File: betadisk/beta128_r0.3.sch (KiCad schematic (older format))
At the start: 85 parts, among them J1 ZX_Spectrum_Connector_GENERIC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, J2 Conn_02x17_Odd_Even, Q1 BC639, SW1 SW_DIP_x02, U10 74LS174, U11 74LS367, U12 FDC_MB8877, U13 74LS14, U14 74LS139, U15 74LS06, U16 74LS74, U17 74LS161, U18 74LS161, U19 74LS00, U21 L7805, U22 GAL22V10, U3 W27C512, U4 74LS32, U6 74LS30, U7 74LS123, U8 74LS74, U9 74LS07, U99 74LS245, Y1 8.000Mhz

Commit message: schematic in pdf
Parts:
- removed C1, C103, C104, C106, C107, C108, C109, C110, C111, C112, C113, C114, C115, C116, C117, C118, C119, C122, C199, C4, C5: 100n, Capacitor_THT:C_Disc_D5.0mm_W2.5mm_P5.00mm, symbol Device:C
- removed C2, C3: 220u/16 V, Capacitor_THT:CP_Radial_D7.5mm_P2.50mm, symbol Device:CP
- removed C6: 10u/16 V, Capacitor_THT:CP_Radial_D7.5mm_P2.50mm, symbol Device:CP
- removed C7: 33p, Capacitor_THT:C_Disc_D5.0mm_W2.5mm_P5.00mm, symbol Device:C
- removed C8: 100u/16 V, Capacitor_THT:CP_Radial_D7.5mm_P2.50mm, symbol Device:CP
- removed D1, D5: LED, LED_THT:LED_D5.0mm, symbol Device:LED
- removed D15: BAT42, Diode_THT:D_DO-35_SOD27_P7.62mm_Horizontal, symbol Diode:BAT42
- removed D7, D8, D9: 1N4148, Diode_THT:D_DO-35_SOD27_P7.62mm_Horizontal, symbol Diode:1N4148
- removed H1, H2, H3, H4: MountingHole, MountingHole:MountingHole_3mm, symbol Mechanical:MountingHole
- removed J1: ZX_Spectrum_Connector_GENERIC_SORTED, SINCLAIR:ZX_EDGE_90extend, symbol 8bits:ZX_Spectrum_Connector_GENERIC_SORTED
- removed J2: Conn_02x17_Odd_Even, Connector_PinHeader_2.54mm:PinHeader_2x17_P2.54mm_Vertical, symbol Connector_Generic:Conn_02x17_Odd_Even
- removed JP2: Conn_01x03, Connector_PinHeader_2.54mm:PinHeader_1x03_P2.54mm_Vertical, symbol Connector_Generic:Conn_01x03
- removed JP3: a, Connector_PinHeader_2.54mm:PinHeader_2x02_P2.54mm_Vertical, symbol Connector_Generic:Conn_02x02_Odd_Even
- removed JP4: Conn_02x02_Odd_Even, Connector_PinHeader_2.54mm:PinHeader_2x02_P2.54mm_Vertical, symbol Connector_Generic:Conn_02x02_Odd_Even
- removed JP5: Conn_01x04_Male, Connector_PinHeader_2.54mm:PinHeader_1x05_P2.54mm_Vertical, symbol Connector:Conn_01x05_Male
- removed Q1: BC639, symbol Device:Q_NPN_ECB
- removed R1: 1k, Resistor_THT:R_Axial_DIN0207_L6.3mm_D2.5mm_P7.62mm_Horizontal, symbol Device:R
- removed R11, R12: 10K, Resistor_THT:R_Axial_DIN0207_L6.3mm_D2.5mm_P7.62mm_Horizontal, symbol Device:R
- removed R13, R14, R15, R16, R17, R3: 470, Resistor_THT:R_Axial_DIN0207_L6.3mm_D2.5mm_P7.62mm_Horizontal, symbol Device:R
- removed R18, R21, R22: 6k8, Resistor_THT:R_Axial_DIN0207_L6.3mm_D2.5mm_P7.62mm_Horizontal, symbol Device:R
- removed R19, R20: 2K2, Resistor_THT:R_Axial_DIN0207_L6.3mm_D2.5mm_P7.62mm_Horizontal, symbol Device:R
- removed R2, R5: 5k6, Resistor_THT:R_Axial_DIN0207_L6.3mm_D2.5mm_P7.62mm_Horizontal, symbol Device:R
- removed R6: 120k, Resistor_THT:R_Axial_DIN0207_L6.3mm_D2.5mm_P7.62mm_Horizontal, symbol Device:R
- removed R8, R9: 680, Resistor_THT:R_Axial_DIN0207_L6.3mm_D2.5mm_P7.62mm_Horizontal, symbol Device:R
- removed S1: 255SB, SINCLAIR:SW_C&K_710x-xx-xx-Z-_SPDT, symbol beta128_r0.3-rescue:255SB-dos_5-0x-eagle-import
- removed S2: 10-XX, Button_Switch_THT:SW_TH_Tactile_Omron_B3F-10xx, symbol beta128_r0.3-rescue:10-XX-dos_5-0x-eagle-import
- removed SW1: SW_DIP_x02, Button_Switch_THT:SW_DIP_SPSTx02_Slide_9.78x7.26mm_W7.62mm_P2.54mm, symbol Switch:SW_DIP_x02
- removed U10: 74LS174, Package_DIP:DIP-16_W7.62mm_LongPads, symbol 74xx:74LS174
- removed U11: 74LS367, Package_DIP:DIP-16_W7.62mm_LongPads, symbol 74xx:74LS367
- removed U12: FDC_MB8877, Package_DIP:DIP-40_W15.24mm_LongPads, symbol 8bits:FDC_MB8877
- removed U13: 74LS14, Package_DIP:DIP-14_W7.62mm_LongPads, symbol 74xx:74LS14
- removed U14: 74LS139, Package_DIP:DIP-16_W7.62mm_LongPads, symbol 74xx:74LS139
- removed U15: 74LS06, Package_DIP:DIP-14_W7.62mm_LongPads, symbol 74xx:74LS06
- removed U16, U8: 74LS74, Package_DIP:DIP-14_W7.62mm_LongPads, symbol 74xx:74LS74
- removed U17, U18: 74LS161, Package_DIP:DIP-16_W7.62mm_LongPads, symbol 74xx:74LS161
- removed U19: 74LS00, Package_DIP:DIP-14_W7.62mm_LongPads, symbol 74xx:74LS00
- removed U21: L7805, Package_TO_SOT_THT:TO-220-3_Vertical, symbol Regulator_Linear:L7805
- removed U22: GAL22V10, Package_DIP:DIP-24_W7.62mm_LongPads, symbol 8bits:GAL22V10
- removed U3: W27C512, Package_DIP:DIP-28_W15.24mm_LongPads, symbol 8bits:W27C512
- removed U4: 74LS32, Package_DIP:DIP-14_W7.62mm_LongPads, symbol 74xx:74LS32
- removed U6: 74LS30, Package_DIP:DIP-14_W7.62mm_LongPads, symbol 74xx:74LS30
- removed U7: 74LS123, Package_DIP:DIP-16_W7.62mm_LongPads, symbol 74xx:74LS123
- removed U9: 74LS07, Package_DIP:DIP-14_W7.62mm_LongPads, symbol 74xx:74LS07
- removed U99: 74LS245, Package_DIP:DIP-20_W7.62mm_LongPads, symbol 74xx:74LS245
- removed Y1: 8.000Mhz, Crystal:Crystal_HC18-U_Vertical, symbol Device:Crystal
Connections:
- net labels removed: +5V, +9V, 4Mhz, A0, A1, A10, A11, A12, A13, A14, A14+A15, A15, A2, A3, A4, A5, A6, A7, A8, A9, A[0...15], D'0, D'1, D'2, D'3, D'4, D'5, D'6, D'7, D'[0...7], D0, D1, D2, D3, D4, D5, D6, D7, DATA_READ, DDEN, DIR, DRQ, DS0, DS1, DS2, DS3, D[0...7], FDC_CS, FDC_IP, FDC_RESET, FDC_TR00, FDC_WPRT, FD_CLK, FD_DATA, GND, HEAD, HLT, INTRQ, IO_WR1, MOTOR_ON, ROM_A14, ROM_A15, ROM_CE, STEP, U10_CP, U11_OEB, U8B_Q, plus3_5V, /(A14+A15), /A9, /IORQ, /IORQ_EXT, /IP, /M1, /MREQ, /NMI, /RD, /RESET, /ROMCS, /ROM_CE, /TR00, /WF, /WPRT, /WR
- wire segments 579 -> 0
- no-connect marks 44 -> 0
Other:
- note removed: "/(A14+A15) = /(A14 * A15)"
- note removed: "/A9 = /A9"
- note removed: "A14&A15 = A14 * A15"
- note removed: "DATA_READ"
- note removed: "DATA_WRITE\n"
- note removed: "DENSITY SEL\n"
- note removed: "DIR = RD + ROM_CE + U8B_Q + /IORQ"
- note removed: "DS0"
- note removed: "DS0\n"
- note removed: "DS1\n"
- note removed: "DS2"
- note removed: "DS3"
- note removed: "FDC_CS = /(A0 + A1) + U8B_Q + /IOREQ + /A7"
- note removed: "GATE_WRITE\n"
- note removed: "INDEX"
- note removed: "IO_WR1= A1+A15+/WR+/IORQ"
- note removed: "MODO XT: 2-3, 4-5 (Cable plano, disqueteras DS0, DS1,hasta 4 unidades)\nMODO AT.: 1-2, 3-4 (Cable cruzado, ambas disqueteras DS1, max 2 unidades)"
- note removed: "MOTOR"
- note removed: "MOTOR 0"
- note removed: "MOTOR 1"
- note removed: "N/C"
- note removed: "READY / Disc Chan."
- note removed: "ROM_CE = /(U8B_Q + A14 + A15 + /RD)"
- note removed: "ROM_CE = U8B_Q + A14 + A15 + /RD"
- note removed: "TRACK 0"
- note removed: "U10_CP = /(A0 + A1) + U8B_Q + /IOREQ + A7 + /RD"
- note removed: "U11_OEB = /(A0 + A1) + U8B_Q + /IOREQ + A7 + /WR"
- note removed: "WRITE PROT"
- note removed: "normal: 1 y 2, 3 y 4, - DS0 es DS0 y DS1 es DS1\ninvertido: 1 y 3, 2 y 4 - DS0 es DS1 DS1 es DS0"

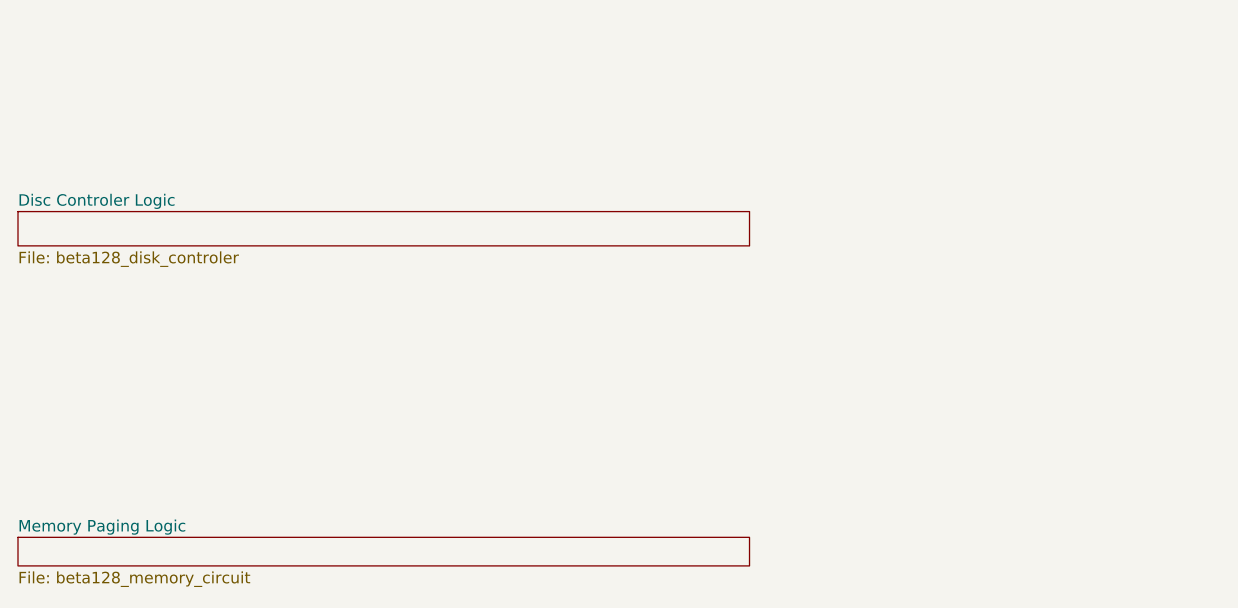
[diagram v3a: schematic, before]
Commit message: update gal code
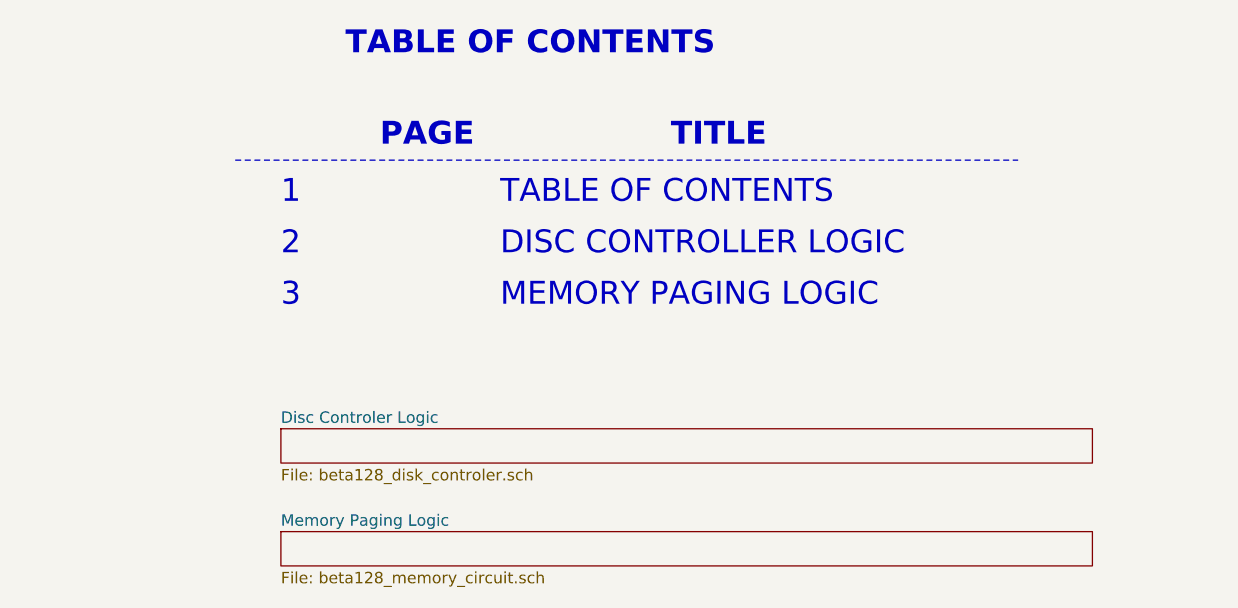
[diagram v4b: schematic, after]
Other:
- note added: "1 TABLE OF CONTENTS"
- note added: "2 DISC CONTROLLER LOGIC"
- note added: "3 MEMORY PAGING LOGIC"
- note added: "PAGE TITLE"
- note added: "TABLE OF CONTENTS"
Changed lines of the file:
@@
 Sheet 1 3
 Title "Beta Disk Interface"
-Date "2020-02-22"
-Rev "0.0"
+Date "2020-03-13"
+Rev "0.3"
 Comp "Alvaro Alea Fdz."
 Comment1 "Based on Rev 5 (Beta 128)"
@@
 Comment9 ""
 $EndDescr
+Wire Notes Line
+	6100 3075 9525 3075
+Text Notes 6300 3275 0    100  ~ 0
+1                    TABLE OF CONTENTS
+Text Notes 6300 3500 0    100  ~ 0
+2                    DISC CONTROLLER LOGIC
+Text Notes 6300 3725 0    100  ~ 0
+3                    MEMORY PAGING LOGIC
+Text Notes 8200 2625 2    100  ~ 20
+TABLE OF CONTENTS
+Text Notes 8425 3025 2    100  ~ 20
+PAGE                  TITLE
 $Sheet
-S 5150 3300 3200 150
+S 6300 4250 3550 150
 U 5E6BCEF8
 F0 "Disc Controler Logic" 50
-F1 "beta128_disk_controler" 50
+F1 "beta128_disk_controler.sch" 50
 $EndSheet
 $Sheet
-S 5150 4725 3200 125
+S 6300 4700 3550 150
 U 5E82F334
 F0 "Memory Paging Logic" 50
-F1 "beta128_memory_circuit" 50
+F1 "beta128_memory_circuit.sch" 50
 $EndSheet
 $EndSCHEMATC
